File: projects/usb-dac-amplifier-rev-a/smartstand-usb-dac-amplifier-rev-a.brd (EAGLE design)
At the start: 174.7 x 136 mm, 226 parts, among them J1 PJ-002A, J2 292304-1, J3 NRJ6HH, J4 PJRAN2X1U01AUX, J5 T1M-5POS, U1 XUF208-256-TQ64, U10 TPS3702, U11 PCM5102A, U12 SZNUD3124, U13 NJM2068M, U14 NJM4556AM, U15 NJM4556AM, U16 TS5A3159DBV, U17 SN74LVC3G34DCU, U18 TPD2E007DCK, U19 TPD2E007DCK, U2 TPD4E02B04DQA, U3 TPS563200DDC, U4 TPS7A8300RGW, U5 TPS563200DDC, U6 TPS7A8300RGW, U7 TPS7A8300RGW, U8 TPS7A4701RGW, U9 TPS7A3301RGW, X1 24MHz, X2 22.5792MHz, X3 24.576MHz

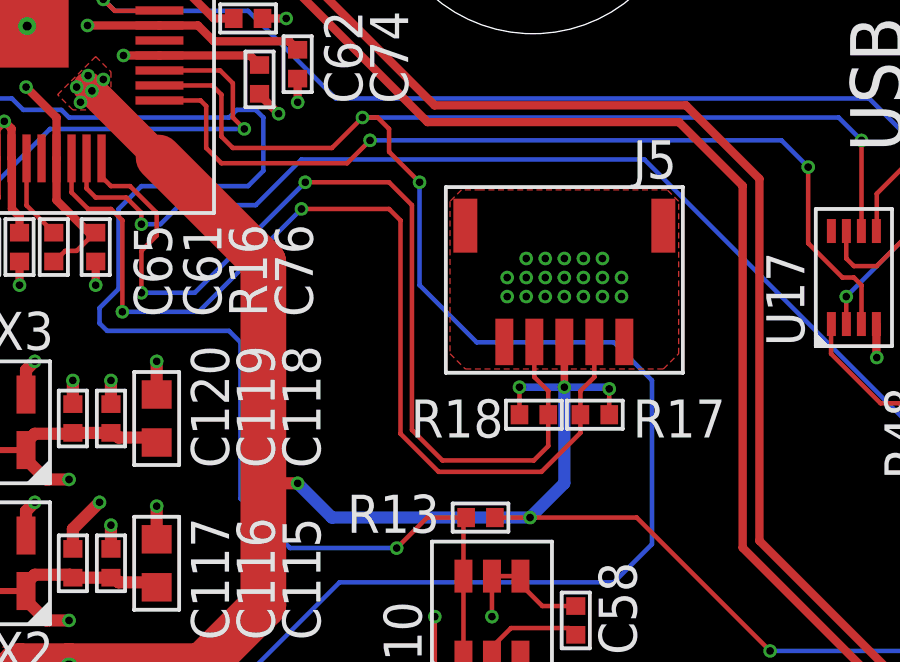
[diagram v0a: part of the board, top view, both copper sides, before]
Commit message: Adjust the I2C pinout on the daughterboard connector.
This will let us have cleaner routing on the small daughterboard which
houses the proximity sensor.
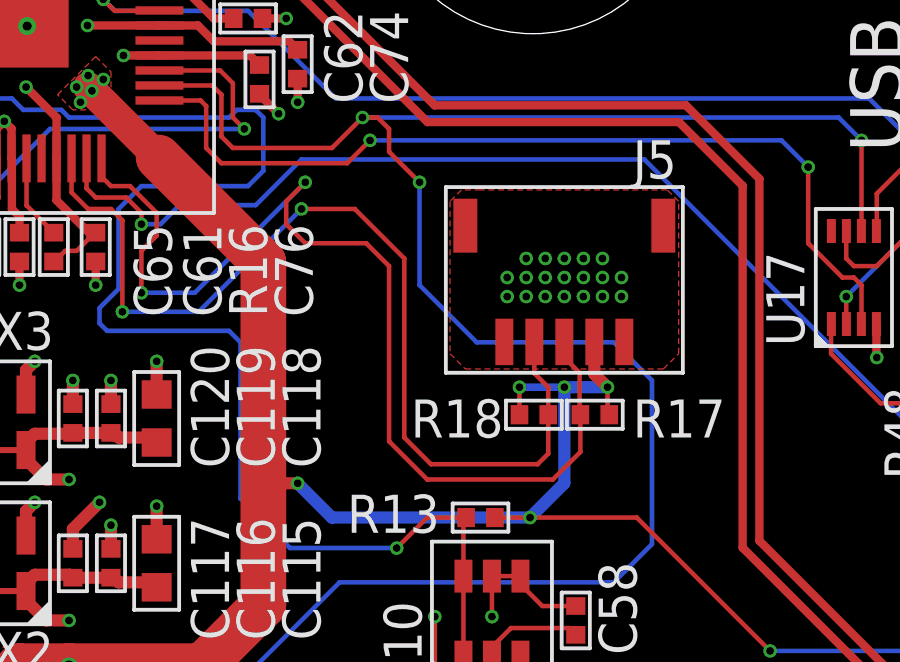
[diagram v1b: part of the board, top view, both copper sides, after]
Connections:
- net DVDD: now also J5.2; no longer J5.3
- net I2C_SCL: now also J5.4, R18.1; no longer J5.2, R17.1
- net I2C_SDA: now also J5.3, R17.1; no longer J5.4, R18.1
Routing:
- net I2C_SDA: track 33.1 -> 35.5 mm
- net I2C_SCL: track 34.6 -> 33.0 mm
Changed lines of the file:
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@@
 <class number="0" name="default" width="0.1524" drill="0.254">
 </class>
-<class number="1" name="USB" width="0.3048" drill="0.254">
+<class number="1" name="USB" width="0.2794" drill="0.254">
 </class>
 </classes>
-<designrules name="OSHPark-4layer">
+<designrules name="OSHPark-4Layer">
 <description language="de">&lt;b&gt;EAGLE Design Rules&lt;/b&gt;
 &lt;p&gt;
@@
 <wire x1="42.799" y1="-20.193" x2="42.799" y2="-12.7" width="1.016" layer="1"/>
 <wire x1="37.084" y1="-6.985" x2="36.957" y2="-6.858" width="1.016" layer="1"/>
-<wire x1="54.328" y1="-17.78" x2="54.328" y2="-16.919" width="0.1524" layer="1"/>
-<via x="54.328" y="-16.919" extent="1-16" drill="0.254"/>
 <via x="43.942" y="-20.066" extent="1-16" drill="0.254"/>
 <wire x1="43.942" y1="-20.066" x2="42.926" y2="-20.066" width="0.4064" layer="1"/>
@@
 <wire x1="45.085" y1="-21.209" x2="43.942" y2="-20.066" width="0.4064" layer="16"/>
 <wire x1="51.308" y1="-16.891" x2="51.336" y2="-16.863" width="0.254" layer="16"/>
-<wire x1="52.832" y1="-16.863" x2="54.272" y2="-16.863" width="0.254" layer="16"/>
-<wire x1="54.272" y1="-16.863" x2="54.328" y2="-16.919" width="0.1524" layer="16"/>
+<wire x1="52.832" y1="-16.863" x2="54.272" y2="-16.863" width="0.4064" layer="16"/>
 <wire x1="73.152" y1="-10.884" x2="73.152" y2="-10.16" width="0.1524" layer="1"/>
 <wire x1="73.152" y1="-10.16" x2="72.898" y2="-9.906" width="0.1524" layer="1"/>
@@
 <vertex x="36.449" y="-7.62"/>
 </polygon>
-<contactref element="J5" pad="3"/>
-<wire x1="52.832" y1="-15.354" x2="52.832" y2="-16.863" width="0.254" layer="1"/>
 <via x="52.832" y="-16.863" extent="1-16" drill="0.254"/>
 <wire x1="52.832" y1="-16.863" x2="51.336" y2="-16.863" width="0.254" layer="16"/>
@@
 <wire x1="27.975" y1="-2.806" x2="26.658" y2="-2.806" width="0.2794" layer="1"/>
 <wire x1="26.658" y1="-2.806" x2="26.543" y2="-2.921" width="0.2794" layer="1"/>
+<contactref element="J5" pad="2"/>
+<via x="54.272" y="-16.863" extent="1-16" drill="0.254"/>
+<wire x1="54.272" y1="-16.863" x2="54.272" y2="-17.724" width="0.1524" layer="1"/>
+<wire x1="54.272" y1="-17.724" x2="54.328" y2="-17.78" width="0.1524" layer="1"/>
+<wire x1="53.832" y1="-15.354" x2="53.832" y2="-16.423" width="0.4064" layer="1"/>
+<wire x1="53.832" y1="-16.423" x2="54.272" y2="-16.863" width="0.4064" layer="1"/>
 </signal>
 <signal name="+1V4">
@@
 <signal name="I2C_SDA">
 <contactref element="U1" pad="P$16"/>
-<contactref element="R18" pad="1"/>
-<contactref element="J5" pad="4"/>
-<wire x1="51.816" y1="-15.37" x2="51.832" y2="-15.354" width="0.1524" layer="1"/>
-<wire x1="52.324" y1="-17.808" x2="52.296" y2="-17.78" width="0.1524" layer="1"/>
-<wire x1="52.324" y1="-17.752" x2="52.296" y2="-17.78" width="0.1524" layer="1"/>
-<wire x1="52.296" y1="-17.78" x2="52.296" y2="-18.824" width="0.1524" layer="1"/>
-<wire x1="52.296" y1="-18.824" x2="51.816" y2="-19.304" width="0.1524" layer="1"/>
-<wire x1="47.752" y1="-18.288" x2="47.752" y2="-10.795" width="0.1524" layer="1"/>
-<wire x1="47.752" y1="-10.795" x2="46.99" y2="-10.033" width="0.1524" layer="1"/>
-<wire x1="46.99" y1="-10.033" x2="44.196" y2="-10.033" width="0.1524" layer="1"/>
 <via x="44.196" y="-10.033" extent="1-16" drill="0.254"/>
 <wire x1="37.405" y1="-9.236" x2="37.405" y2="-9.846" width="0.1524" layer="1"/>
@@
 <via x="38.735" y="-13.716" extent="1-16" drill="0.254"/>
 <wire x1="40.513" y1="-13.716" x2="44.196" y2="-10.033" width="0.1524" layer="16"/>
-<wire x1="52.296" y1="-17.78" x2="52.296" y2="-16.99" width="0.1524" layer="1"/>
-<wire x1="52.296" y1="-16.99" x2="51.832" y2="-16.526" width="0.1524" layer="1"/>
-<wire x1="51.832" y1="-15.354" x2="51.832" y2="-16.526" width="0.1524" layer="1"/>
 <wire x1="38.735" y1="-13.716" x2="40.513" y2="-13.716" width="0.1524" layer="16"/>
 <wire x1="38.354" y1="-10.16" x2="39.243" y2="-11.049" width="0.1524" layer="1"/>
 <wire x1="39.243" y1="-11.049" x2="39.243" y2="-11.811" width="0.1524" layer="1"/>
 <wire x1="39.243" y1="-11.811" x2="38.735" y2="-12.319" width="0.1524" layer="1"/>
-<wire x1="51.816" y1="-19.304" x2="48.768" y2="-19.304" width="0.1524" layer="1"/>
-<wire x1="48.768" y1="-19.304" x2="47.752" y2="-18.288" width="0.1524" layer="1"/>
+<contactref element="J5" pad="3"/>
+<contactref element="R17" pad="1"/>
+<wire x1="52.832" y1="-15.354" x2="52.832" y2="-15.875" width="0.1524" layer="1"/>
+<wire x1="52.832" y1="-15.875" x2="53.34" y2="-16.383" width="0.1524" layer="1"/>
+<wire x1="53.34" y1="-16.383" x2="53.34" y2="-17.752" width="0.1524" layer="1"/>
+<wire x1="53.34" y1="-17.752" x2="53.368" y2="-17.78" width="0.1524" layer="1"/>
+<wire x1="44.196" y1="-10.033" x2="43.561" y2="-10.668" width="0.1524" layer="1"/>
+<wire x1="43.561" y1="-10.668" x2="43.561" y2="-11.43" width="0.1524" layer="1"/>
+<wire x1="43.561" y1="-11.43" x2="44.196" y2="-12.065" width="0.1524" layer="1"/>
+<wire x1="44.196" y1="-12.065" x2="46.228" y2="-12.065" width="0.1524" layer="1"/>
+<wire x1="46.228" y1="-12.065" x2="46.99" y2="-12.827" width="0.1524" layer="1"/>
+<wire x1="46.99" y1="-12.827" x2="46.99" y2="-18.669" width="0.1524" layer="1"/>
+<wire x1="46.99" y1="-18.669" x2="48.26" y2="-19.939" width="0.1524" layer="1"/>
+<wire x1="48.26" y1="-19.939" x2="52.451" y2="-19.939" width="0.1524" layer="1"/>
+<wire x1="52.451" y1="-19.939" x2="53.368" y2="-19.022" width="0.1524" layer="1"/>
+<wire x1="53.368" y1="-17.78" x2="53.368" y2="-19.022" width="0.1524" layer="1"/>
 </signal>
 <signal name="I2C_SCL">
 <contactref element="U1" pad="P$14"/>
-<contactref element="R17" pad="1"/>
-<contactref element="J5" pad="2"/>
-<wire x1="53.848" y1="-15.37" x2="53.832" y2="-15.354" width="0.1524" layer="1"/>
-<wire x1="53.34" y1="-17.752" x2="53.368" y2="-17.78" width="0.1524" layer="1"/>
-<wire x1="53.368" y1="-17.78" x2="53.368" y2="-18.387" width="0.1524" layer="1"/>
-<wire x1="53.368" y1="-18.387" x2="52.07" y2="-19.685" width="0.1524" layer="1"/>
-<wire x1="52.07" y1="-19.685" x2="48.641" y2="-19.685" width="0.1524" layer="1"/>
-<wire x1="47.371" y1="-18.415" x2="47.371" y2="-11.303" width="0.1524" layer="1"/>
-<wire x1="47.371" y1="-11.303" x2="46.99" y2="-10.922" width="0.1524" layer="1"/>
-<wire x1="46.99" y1="-10.922" x2="44.069" y2="-10.922" width="0.1524" layer="1"/>
 <via x="44.069" y="-10.922" extent="1-16" drill="0.254"/>
 <wire x1="36.405" y1="-9.236" x2="36.405" y2="-10.37" width="0.1524" layer="1"/>
@@
 <via x="38.1" y="-14.351" extent="1-16" drill="0.254"/>
 <wire x1="40.64" y1="-14.351" x2="44.069" y2="-10.922" width="0.1524" layer="16"/>
-<wire x1="53.368" y1="-17.78" x2="53.368" y2="-16.99" width="0.1524" layer="1"/>
-<wire x1="53.368" y1="-16.99" x2="53.832" y2="-16.526" width="0.1524" layer="1"/>
-<wire x1="53.832" y1="-15.354" x2="53.832" y2="-16.526" width="0.1524" layer="1"/>
 <wire x1="38.1" y1="-14.351" x2="40.64" y2="-14.351" width="0.1524" layer="16"/>
-<wire x1="48.641" y1="-19.685" x2="47.371" y2="-18.415" width="0.1524" layer="1"/>
+<contactref element="J5" pad="4"/>
+<contactref element="R18" pad="1"/>
+<wire x1="51.832" y1="-15.354" x2="51.832" y2="-16.399" width="0.1524" layer="1"/>
+<wire x1="51.832" y1="-16.399" x2="52.296" y2="-16.863" width="0.1524" layer="1"/>
+<wire x1="52.296" y1="-17.78" x2="52.296" y2="-16.863" width="0.1524" layer="1"/>
+<wire x1="44.069" y1="-10.922" x2="45.847" y2="-10.922" width="0.1524" layer="1"/>
+<wire x1="45.847" y1="-10.922" x2="47.498" y2="-12.573" width="0.1524" layer="1"/>
+<wire x1="47.498" y1="-12.573" x2="47.498" y2="-18.542" width="0.1524" layer="1"/>
+<wire x1="47.498" y1="-18.542" x2="48.387" y2="-19.431" width="0.1524" layer="1"/>
+<wire x1="48.387" y1="-19.431" x2="51.943" y2="-19.431" width="0.1524" layer="1"/>
+<wire x1="52.296" y1="-17.78" x2="52.296" y2="-19.078" width="0.1524" layer="1"/>
+<wire x1="52.296" y1="-19.078" x2="51.943" y2="-19.431" width="0.1524" layer="1"/>
 </signal>
 <signal name="JACK_ENABLE">
